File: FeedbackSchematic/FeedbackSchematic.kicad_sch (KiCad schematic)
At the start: 102 parts, among them J1 Screw_Terminal_01x02, J10 Conn_01x02_Male, J11 Conn_01x02_Male, J2 Screw_Terminal_01x08, J3 Conn_01x08_Male, J4 Conn_01x08_Male, J5 Conn_01x08_Male, J6 RJ45, J7 RJ45, J8 Conn_01x04_Male, J9 Conn_01x03_Male, U1 BluePill_STM32F103C, U2 L7805, U3 L7805, U4 6N137, U5 6N137, U6 TJA1050_Board, U7 74HC595, U8 74HC595

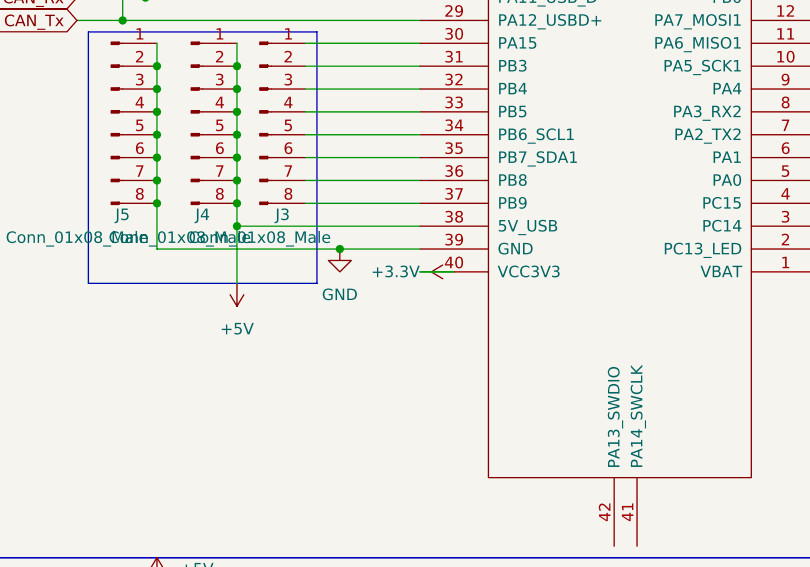
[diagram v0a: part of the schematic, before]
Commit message: Updated footprint
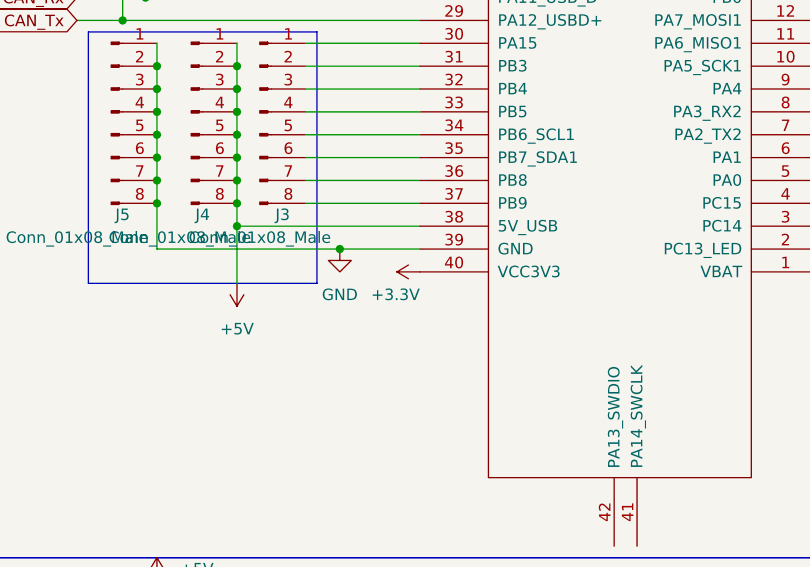
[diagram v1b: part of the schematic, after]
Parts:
- J1: footprint TerminalBlock_RND:TerminalBlock_RND_205-00002_1x03_P5.00mm_Horizontal -> TerminalBlock_RND:TerminalBlock_RND_205-00012_1x02_P5.00mm_Horizontal
- U1: footprint BluePill_breakouts:BluePill_STM32F103C -> Footprint_Marcel:Bluepill
- U6: footprint (none) -> Footprint_Marcel:TJA1050
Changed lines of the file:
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@@
     (stroke (width 0) (type default) (color 0 0 0 0))
   )
-  (wire (pts (xy 68.58 120.65) (xy 64.77 120.65))
-    (stroke (width 0) (type default) (color 0 0 0 0))
-  )
   (wire (pts (xy 55.88 186.69) (xy 85.09 186.69))
     (stroke (width 0) (type default) (color 0 0 0 0))
@@
     (property "Reference" "U1" (id 0) (at 86.995 62.23 0))
     (property "Value" "BluePill_STM32F103C" (id 1) (at 86.995 64.77 0))
-    (property "Footprint" "BluePill_breakouts:BluePill_STM32F103C" (id 2) (at 86.36 62.23 0)
+    (property "Footprint" "Footprint_Marcel:Bluepill" (id 2) (at 86.36 62.23 0)
       (effects (font (size 1.27 1.27)) hide)
     )
@@
     (property "Reference" "U6" (id 0) (at 231.14 111.76 0))
     (property "Value" "TJA1050_Board" (id 1) (at 231.14 114.3 0))
-    (property "Footprint" "" (id 2) (at 231.14 115.57 0)
+    (property "Footprint" "Footprint_Marcel:TJA1050" (id 2) (at 231.14 115.57 0)
       (effects (font (size 1.27 1.27)) hide)
     )
@@
       (effects (font (size 1.27 1.27)) (justify left))
     )
-    (property "Footprint" "TerminalBlock_RND:TerminalBlock_RND_205-00002_1x03_P5.00mm_Horizontal" (id 2) (at 22.86 25.4 0)
+    (property "Footprint" "TerminalBlock_RND:TerminalBlock_RND_205-00012_1x02_P5.00mm_Horizontal" (id 2) (at 22.86 25.4 0)
       (effects (font (size 1.27 1.27)) hide)
     )
@@
     (pin "2")
   )
-  (symbol (lib_id "power:+3.3V") (at 68.58 120.65 90) (unit 1)
-    (in_bom yes) (on_board yes) (fields_autoplaced)
-    (property "Reference" "#PWR04" (id 0) (at 72.39 120.65 0)
+  (symbol (lib_id "power:+3.3V") (at 64.77 120.65 90) (unit 1)
+    (in_bom yes) (on_board yes)
+    (property "Reference" "#PWR04" (id 0) (at 68.58 120.65 0)
       (effects (font (size 1.27 1.27)) hide)
     )
-    (property "Value" "+3.3V" (id 1) (at 64.77 120.6499 90)
+    (property "Value" "+3.3V" (id 1) (at 64.77 123.19 90)
       (effects (font (size 1.27 1.27)) (justify left))
     )
-    (property "Footprint" "" (id 2) (at 68.58 120.65 0)
+    (property "Footprint" "" (id 2) (at 64.77 120.65 0)
       (effects (font (size 1.27 1.27)) hide)
     )
-    (property "Datasheet" "" (id 3) (at 68.58 120.65 0)
+    (property "Datasheet" "" (id 3) (at 64.77 120.65 0)
       (effects (font (size 1.27 1.27)) hide)
     )
@@
     )
     (path "/8cf2a6b6-ba53-4401-8b5b-6d344d0b7e0e"
-      (reference "J1") (unit 1) (value "Screw_Terminal_01x02") (footprint "TerminalBlock_RND:TerminalBlock_RND_205-00002_1x03_P5.00mm_Horizontal")
+      (reference "J1") (unit 1) (value "Screw_Terminal_01x02") (footprint "TerminalBlock_RND:TerminalBlock_RND_205-00012_1x02_P5.00mm_Horizontal")
     )
     (path "/f68b0618-192e-4836-84f5-d0253d207d5a"
@@
     )
     (path "/1065cb5f-54ca-45cc-b2ab-e8803f30a939"
-      (reference "U1") (unit 1) (value "BluePill_STM32F103C") (footprint "BluePill_breakouts:BluePill_STM32F103C")
+      (reference "U1") (unit 1) (value "BluePill_STM32F103C") (footprint "Footprint_Marcel:Bluepill")
     )
     (path "/e604f0f9-1111-4069-a4eb-9c5688696bf6"
@@
     )
     (path "/63950369-1610-449f-b07e-5ef80631f63c"
-      (reference "U6") (unit 1) (value "TJA1050_Board") (footprint "")
+      (reference "U6") (unit 1) (value "TJA1050_Board") (footprint "Footprint_Marcel:TJA1050")
     )
     (path "/1ab9b1bd-eda3-477d-a65e-83d660ed9f83"
